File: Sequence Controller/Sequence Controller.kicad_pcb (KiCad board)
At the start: 2 copper layers, 32.8 x 50.7 mm, 13 parts, among them J1 , Q1 BSR202N, Q2 BSR202N, Q3 BSR202N, Q4 BSR202N, Q5 BSR202N, Q6 BSR202N, Q7 BSR202N, Q8 BSR202N, U1 ESP32Devkit30

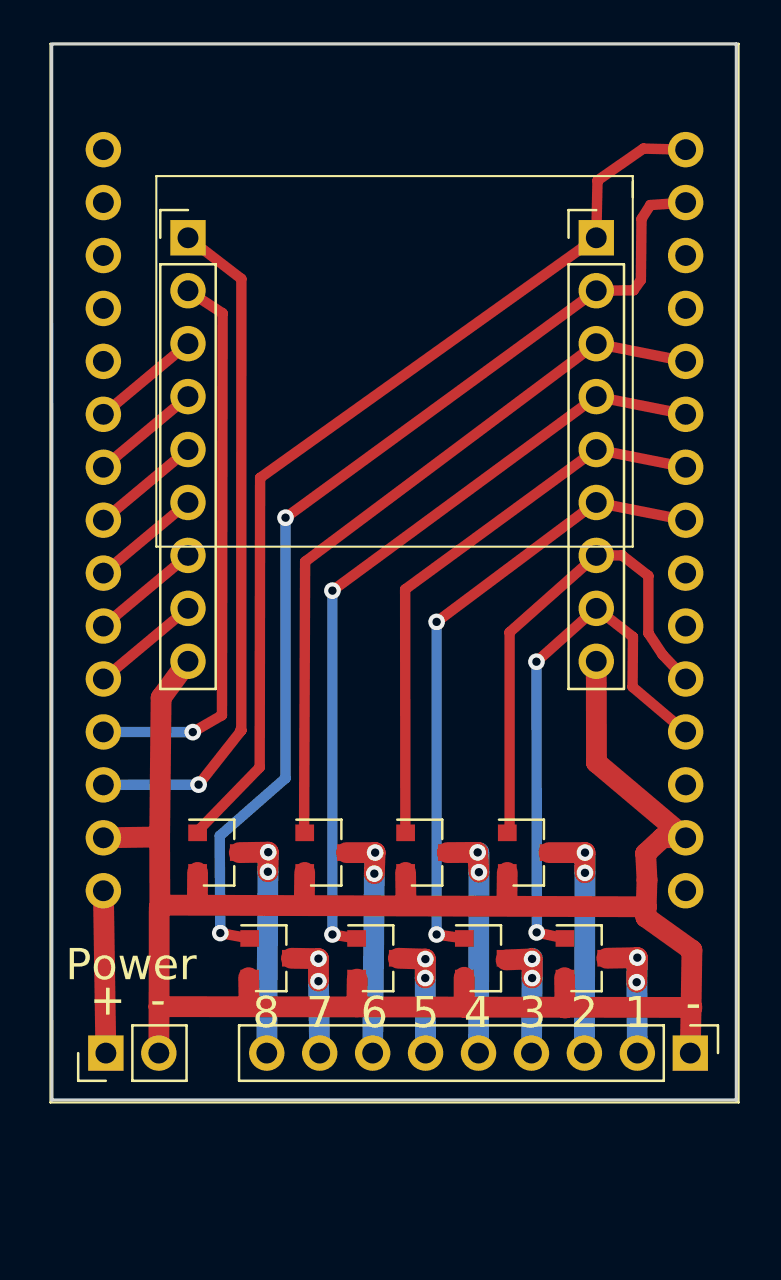
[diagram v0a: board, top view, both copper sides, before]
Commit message: new design, new code
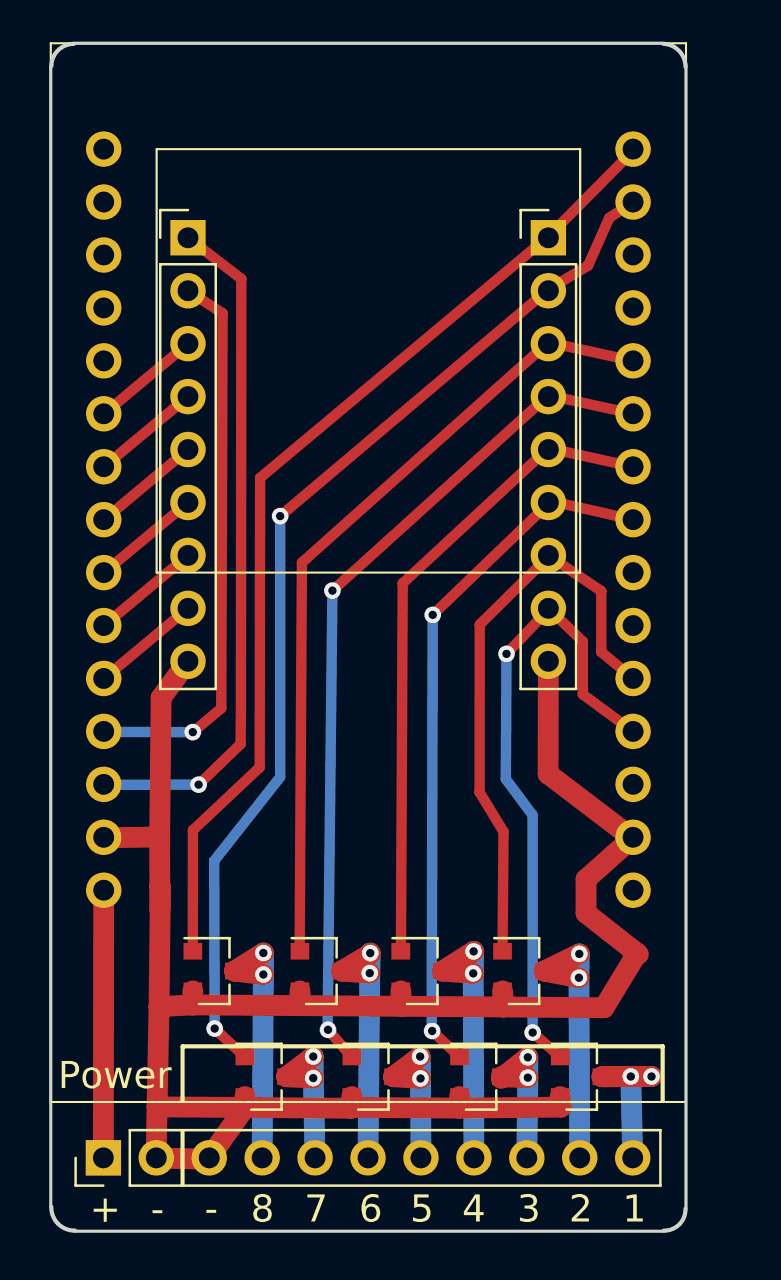
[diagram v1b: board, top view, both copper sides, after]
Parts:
- removed Output1: , Pin_Headers:Pin_Header_Straight_1x09_Pitch2.54mm
- J1: value (none) -> Conn_01x11_Male; footprint Pin_Headers:Pin_Header_Straight_1x02_Pitch2.54mm -> Pin_Headers:Pin_Header_Straight_1x11_Pitch2.54mm
- moved Q1 5.69 mm to (118.1, 115.0)
- moved Q2 5.69 mm to (120.6, 120.1)
- moved Q3 5.69 mm to (123.2, 115.0)
- moved Q4 5.69 mm to (125.7, 120.1)
- moved Q5 5.69 mm to (128.0, 115.0)
- moved Q6 5.69 mm to (130.9, 120.1)
- moved Q7 5.69 mm to (132.9, 115.0)
- moved Q8 5.69 mm to (135.7, 120.1)
- moved J1 5.03 mm to (112.8, 124.0)
- moved U1 2.52 mm to (125.5, 93.3)
- moved ExtIn1 2.30 mm to (134.1, 79.8)
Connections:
- Q1 pad 3: Net-(Output1-Pad9) -> Net-(J1-Pad4)
- Q2 pad 3: Net-(Output1-Pad8) -> Net-(J1-Pad5)
- Q3 pad 3: Net-(Output1-Pad7) -> Net-(J1-Pad6)
- Q4 pad 3: Net-(Output1-Pad6) -> Net-(J1-Pad7)
- Q5 pad 3: Net-(Output1-Pad5) -> Net-(J1-Pad8)
- Q6 pad 3: Net-(Output1-Pad4) -> Net-(J1-Pad9)
- Q7 pad 3: Net-(Output1-Pad3) -> Net-(J1-Pad10)
- Q8 pad 3: Net-(Output1-Pad2) -> Net-(J1-Pad11)
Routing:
- net Net-(J1-Pad10): track 0.00 -> 13.4 mm, vias 0 -> 2
- net Net-(J1-Pad8): track 0.00 -> 13.2 mm, vias 0 -> 2
- net Net-(J1-Pad4): track 0.00 -> 12.9 mm, vias 0 -> 2
- net Net-(J1-Pad6): track 0.00 -> 12.8 mm, vias 0 -> 2
- net Net-(Output1-Pad3): track 12.3 -> 0.00 mm, vias 2 -> 0
- net Net-(Output1-Pad5): track 12.0 -> 0.00 mm, vias 2 -> 0
- net Net-(Output1-Pad9): track 12.0 -> 0.00 mm, vias 2 -> 0
- net Net-(Output1-Pad7): track 11.9 -> 0.00 mm, vias 2 -> 0
- net Net-(J1-Pad11): track 0.00 -> 8.67 mm, vias 0 -> 2
- net Net-(J1-Pad7): track 0.00 -> 7.77 mm, vias 0 -> 2
- net Net-(J1-Pad5): track 0.00 -> 7.75 mm, vias 0 -> 2
- net Net-(J1-Pad9): track 0.00 -> 7.73 mm, vias 0 -> 2
- net Net-(Output1-Pad2): track 7.24 -> 0.00 mm, vias 2 -> 0
- net Net-(Output1-Pad8): track 6.91 -> 0.00 mm, vias 2 -> 0
- net Net-(Output1-Pad4): track 6.72 -> 0.00 mm, vias 2 -> 0
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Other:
- board size 32.8 x 50.7 mm -> 30.5 x 57 mm
